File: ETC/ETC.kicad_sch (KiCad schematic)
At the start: 36 parts, among them P1 DTM1312PC12PDR008, U1 NUCLEO-F446RE, U2 MCP6004, U3 LM7805_TO220, U4 LM7809_TO220, U5 ISO1050DUB, U6 ISO1050DUB, U7 SN74AHC14N

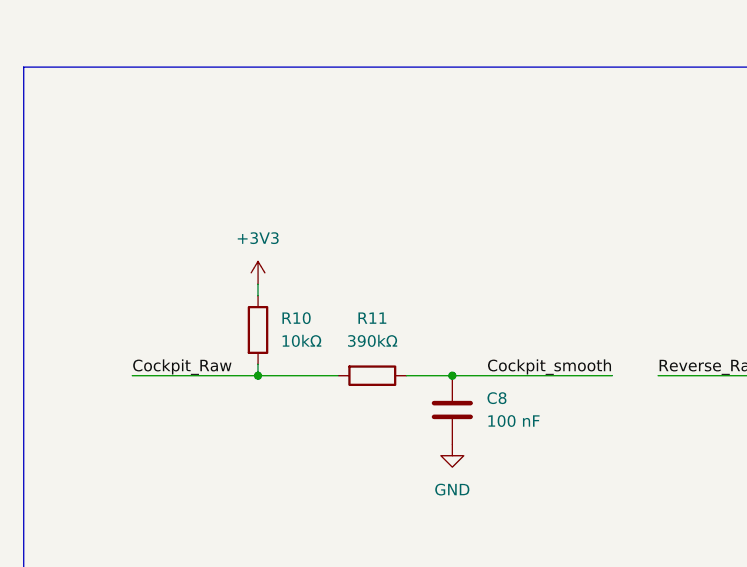
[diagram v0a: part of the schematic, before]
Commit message: NUCLEO F446RE footprint fix
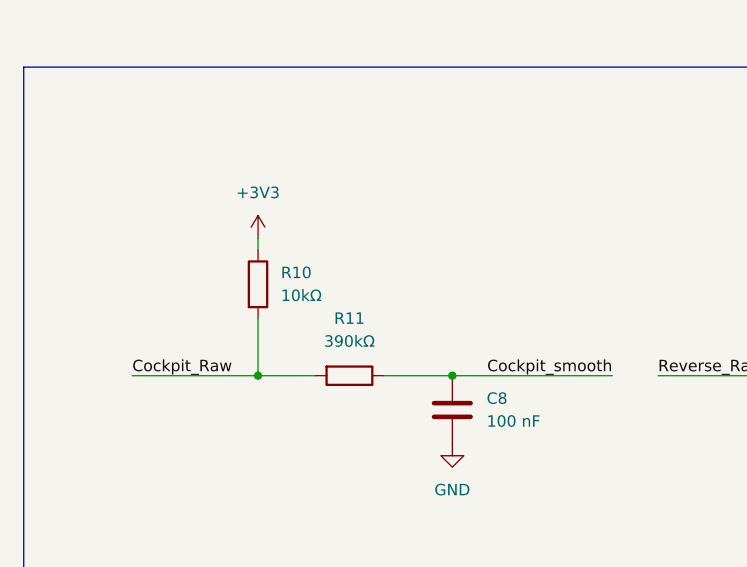
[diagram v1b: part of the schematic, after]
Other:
- moved on the sheet: R10, R11
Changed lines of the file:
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@@
 	(wire
 		(pts
-			(xy 44.45 223.52) (xy 53.34 223.52)
+			(xy 44.45 223.52) (xy 50.8 223.52)
 		)
 		(stroke
@@
 	(wire
 		(pts
-			(xy 44.45 213.36) (xy 44.45 214.63)
+			(xy 44.45 208.28) (xy 44.45 209.55)
+		)
+		(stroke
+			(width 0)
+			(type default)
+		)
+	)
+	(wire
+		(pts
+			(xy 44.45 217.17) (xy 44.45 223.52)
 		)
 		(stroke
@@
 	(wire
 		(pts
-			(xy 44.45 222.25) (xy 44.45 223.52)
-		)
-		(stroke
-			(width 0)
-			(type default)
-		)
-	)
-	(wire
-		(pts
 			(xy 134.62 106.68) (xy 144.78 106.68)
 		)
@@
 	(wire
 		(pts
-			(xy 60.96 223.52) (xy 66.04 223.52)
+			(xy 58.42 223.52) (xy 66.04 223.52)
 		)
 		(stroke
@@
 	(symbol
 		(lib_id "power:+3V3")
-		(at 44.45 213.36 0)
+		(at 44.45 208.28 0)
 		(unit 1)
 		(exclude_from_sim no)
@@
 		(fields_autoplaced yes)
 		(property "Reference" "#PWR029"
-			(at 44.45 217.17 0)
+			(at 44.45 212.09 0)
 			(effects
 				(font
@@
 		)
 		(property "Value" "+3V3"
-			(at 44.45 208.28 0)
+			(at 44.45 203.2 0)
 			(effects
 				(font
@@
 		)
 		(property "Footprint" ""
-			(at 44.45 213.36 0)
+			(at 44.45 208.28 0)
 			(effects
 				(font
@@
 		)
 		(property "Datasheet" ""
-			(at 44.45 213.36 0)
+			(at 44.45 208.28 0)
 			(effects
 				(font
@@
 		)
 		(property "Description" "Power symbol creates a global label with name \"+3V3\""
-			(at 44.45 213.36 0)
+			(at 44.45 208.28 0)
 			(effects
 				(font
@@
 	(symbol
 		(lib_id "Device:R")
-		(at 44.45 218.44 0)
+		(at 44.45 213.36 0)
 		(unit 1)
 		(exclude_from_sim no)
@@
 		(fields_autoplaced yes)
 		(property "Reference" "R10"
-			(at 46.99 217.17 0)
+			(at 46.99 212.09 0)
 			(effects
 				(font
@@
 		)
 		(property "Value" "10kΩ"
-			(at 46.99 219.71 0)
+			(at 46.99 214.63 0)
 			(effects
 				(font
@@
 		)
 		(property "Footprint" "Resistor_SMD:R_0805_2012Metric_Pad1.20x1.40mm_HandSolder"
-			(at 42.672 218.44 90)
+			(at 42.672 213.36 90)
 			(effects
 				(font
@@
 		)
 		(property "Datasheet" "~"
-			(at 44.45 218.44 0)
+			(at 44.45 213.36 0)
 			(effects
 				(font
@@
 		)
 		(property "Description" ""
-			(at 44.45 218.44 0)
+			(at 44.45 213.36 0)
 			(effects
 				(font
@@
 	(symbol
 		(lib_id "Device:R")
-		(at 57.15 223.52 270)
+		(at 54.61 223.52 270)
 		(unit 1)
 		(exclude_from_sim no)
@@
 		(fields_autoplaced yes)
 		(property "Reference" "R11"
-			(at 57.15 217.17 90)
+			(at 54.61 217.17 90)
 			(effects
 				(font
@@
 		)
 		(property "Value" "390kΩ"
-			(at 57.15 219.71 90)
+			(at 54.61 219.71 90)
 			(effects
 				(font
@@
 		)
 		(property "Footprint" "Resistor_SMD:R_0805_2012Metric_Pad1.20x1.40mm_HandSolder"
-			(at 57.15 221.742 90)
+			(at 54.61 221.742 90)
 			(effects
 				(font
@@
 		)
 		(property "Datasheet" "~"
-			(at 57.15 223.52 0)
+			(at 54.61 223.52 0)
 			(effects
 				(font
@@
 		)
 		(property "Description" "Resistor"
-			(at 57.15 223.52 0)
+			(at 54.61 223.52 0)
 			(effects
 				(font
